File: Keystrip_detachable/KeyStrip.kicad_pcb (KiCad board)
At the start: 2 copper layers, 19.1 x 57.2 mm, 19 parts, among them J1 JST_06, J2 JST_08, J3 JST_06, J4 JST_06, J4 JST_08

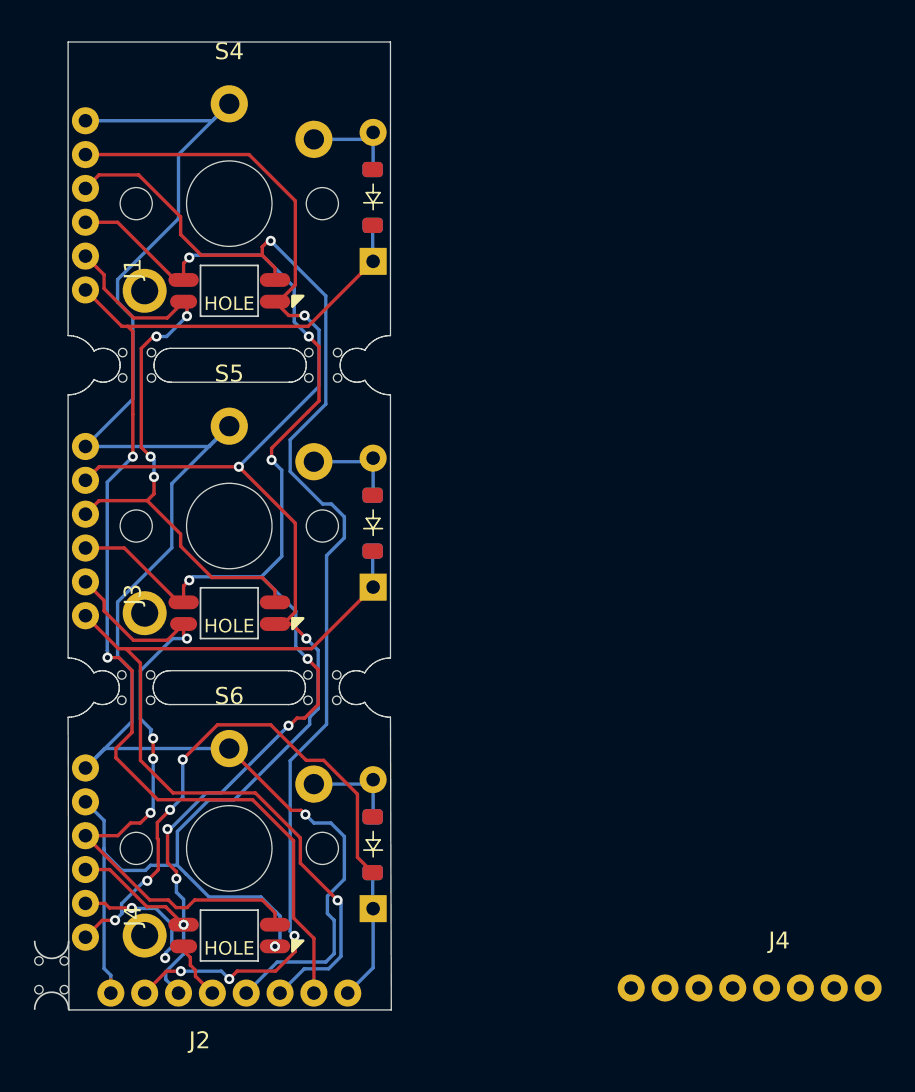
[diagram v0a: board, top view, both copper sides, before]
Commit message: uhhh, This feels both improved and weirder
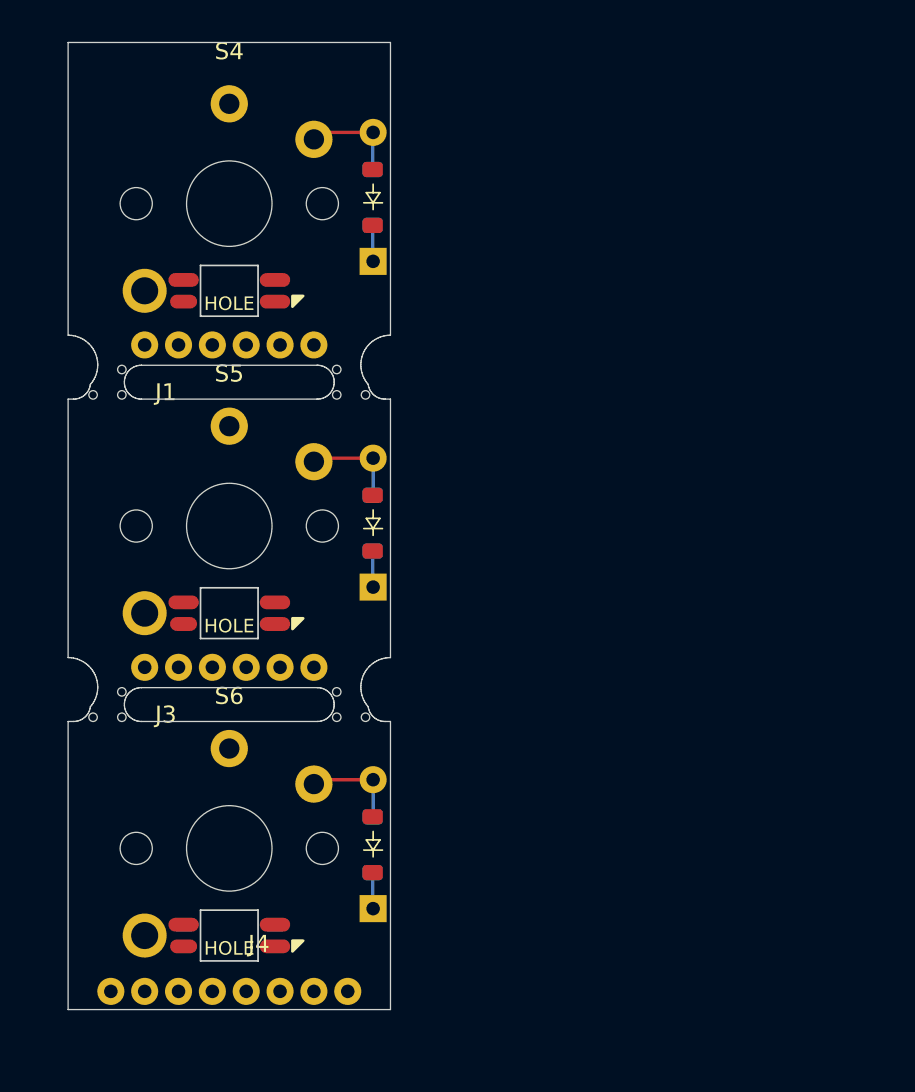
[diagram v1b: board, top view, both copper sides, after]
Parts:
- removed J2: JST_08, Library:JST_EH_B8B-EH-A_1x08_P2.50mm_Vertical
- removed the J4 at (62.8, 102.5)
- removed the REF** at (61.8, 114.8)
- removed the REF** at (76.8, 97.8)
- removed the REF** at (65.8, 97.8)
- removed the REF** at (76.8, 78.7)
- removed the REF** at (65.8, 78.7)
- added ?: , , F.Cu at (77.6, 80.5)
- added ?: , , F.Cu at (63.2, 80.5)
- added ?: , , F.Cu at (63.2, 99.5)
- added ?: , , F.Cu at (64.9, 99.5)
- added ?: , , F.Cu at (79.3, 99.5)
- added ?: , , F.Cu at (64.9, 98.0)
- added ?: , , F.Cu at (79.3, 80.5)
- added ?: , , F.Cu at (64.9, 79.0)
- added ?: , , F.Cu at (64.9, 80.5)
- added ?: , , F.Cu at (77.6, 98.0)
- added ?: , , F.Cu at (77.6, 79.0)
- added REF**: LilHole, Library:LilHole, F.Cu at (77.6, 99.5)
- moved J4 30.8 mm to (64.2, 115.7)
- moved J1 18.9 mm to (76.2, 77.5), turned to 180 degrees
- moved J3 18.8 mm to (76.2, 96.5), turned to 180 degrees
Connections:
- J1 pad 2: /8 -> /7
- J1 pad 3: /7 -> /8
- J1 pad 4: /6 -> Net-(D10-DOUT)
- J1 pad 5: Net-(D10-DOUT) -> /6
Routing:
- net Net-(D10-VSS): track 102.0 -> 0.00 mm, vias 4 -> 0
- net Net-(J1-Pad1): track 98.8 -> 0.00 mm, vias 1 -> 0
- net Net-(D10-VDD): track 87.6 -> 0.00 mm, vias 9 -> 0
- net Net-(D10-DIN): track 73.9 -> 0.00 mm, vias 4 -> 0
- net Net-(D7-K): track 71.3 -> 0.00 mm, vias 2 -> 0
- net Net-(D8-K): track 52.3 -> 0.00 mm, vias 1 -> 0
- net Net-(D11-DOUT): track 39.9 -> 0.00 mm, vias 4 -> 0
- net Net-(D9-K): track 39.1 -> 0.00 mm, vias 4 -> 0
- net Net-(D10-DOUT): track 37.0 -> 0.00 mm, vias 4 -> 0
- net Net-(D12-DOUT): track 11.3 -> 0.00 mm, vias 2 -> 0
- net /3: track 0.00 -> 2.14 mm
- net /2: track 0.00 -> 2.14 mm
- net /1: track 0.00 -> 2.14 mm
- net /7: track 0.00 -> 0.85 mm
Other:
- outline, holes or cut-outs redrawn
- board text removed: "${REFERENCE}"
